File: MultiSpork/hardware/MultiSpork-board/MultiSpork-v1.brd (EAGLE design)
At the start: 86.4 x 76.2 mm, 216 parts, among them J1 U.FL, Q2 32.768 kHz, Q3 40 MHz, Q4 MMBT3904, Q5 MMBT3904, SW1 JS102011SAQN, U1 USD-SOCKETNEW, U10 M25PX80, U2 SAM3SA-MU, U3 MAX11300GTL, U4 LT3580EMS8E, U5 LT3580EMS8E, U6 LT3580EMS8E, U7 MCP73831, U8 LT3580EMS8E, U9 CC3100

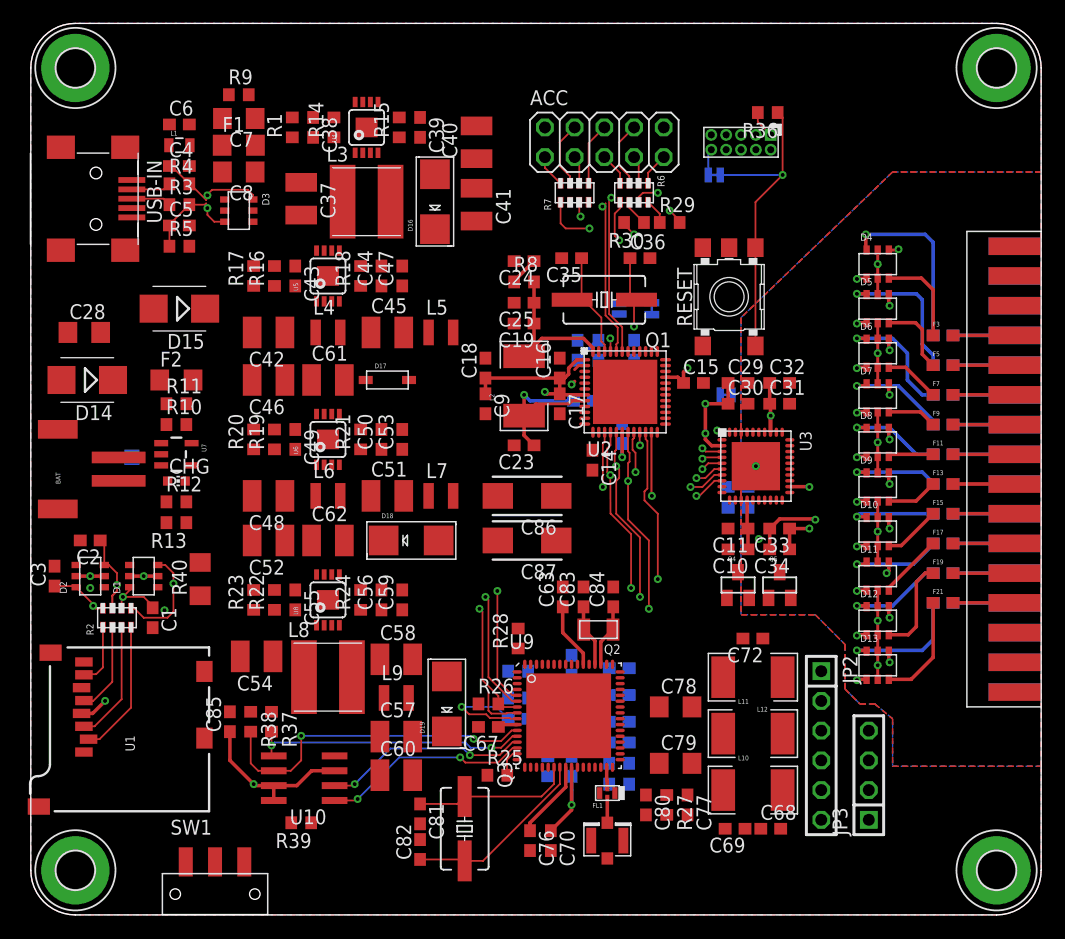
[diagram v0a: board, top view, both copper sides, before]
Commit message: Finished routing
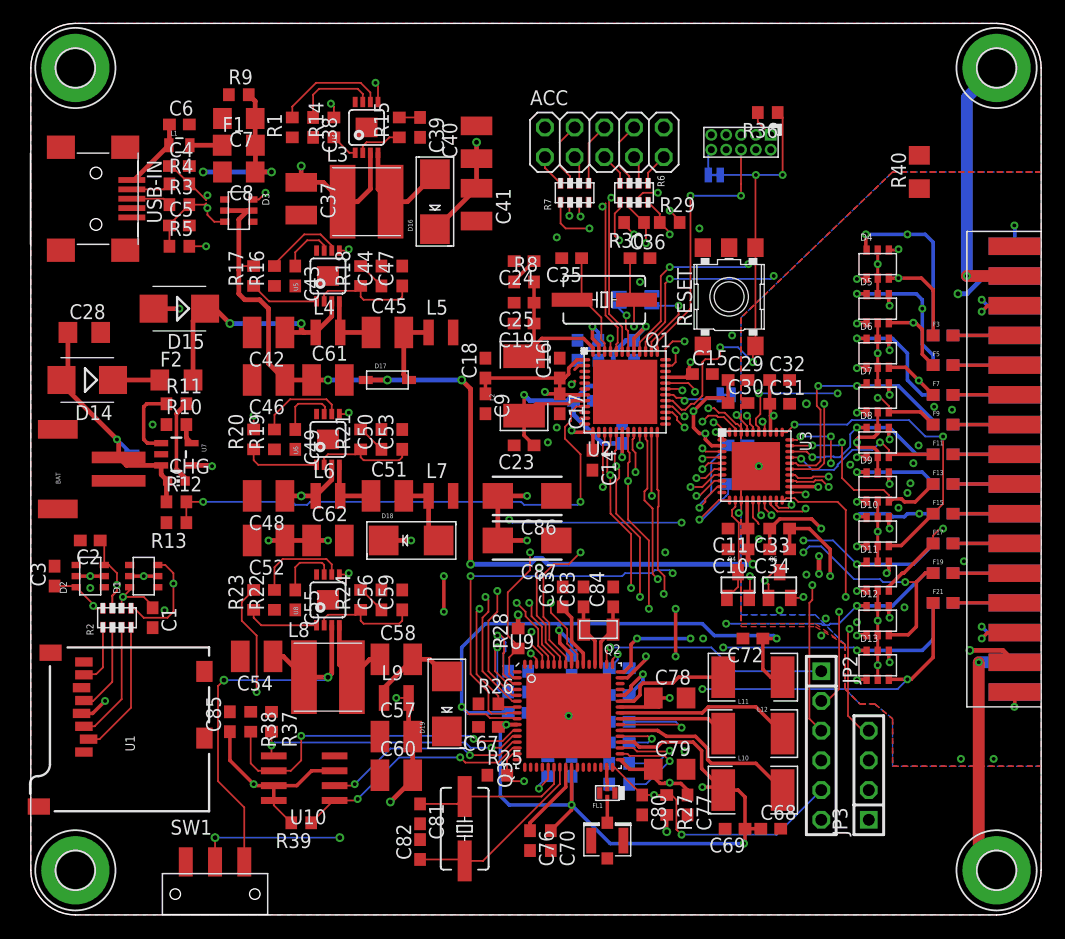
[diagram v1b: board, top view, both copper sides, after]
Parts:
- moved R40 70.6 mm to (75.9, 63.5)
- moved C21 3.56 mm to (60.5, 40.1)
- moved C27 2.03 mm to (60.5, 36.8)
- moved C15 1.08 mm to (57.4, 46.2)
- moved C78 0.92 mm to (54.6, 18.5)
- moved ERASE 0.76 mm to (50.3, 52.6)
- moved JTAGSEL 0.76 mm to (53.1, 52.6)
- moved C79 0.72 mm to (54.6, 12.4)
- moved C73 0.51 mm to (41.7, 17.3)
- moved R31 0.51 mm to (41.7, 19.1)
- moved C80 0.32 mm to (52.3, 9.40)
- moved C29 0.25 mm to (60.5, 45.7)
- moved C32 0.25 mm to (64.0, 45.7)
- moved C30 0.06 mm to (60.5, 43.8)
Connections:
- net N$115 renamed D1P
- net N$116 renamed D1N
- net N$117 renamed D0N
- net N$118 renamed D0P
- net N$19 renamed PLL-GND
- net N$32 renamed ADC_REF
- net N$33 renamed DAC_REF
- net N$34 renamed PORT00'
- net N$35 renamed PORT01'
- net N$36 renamed PORT02'
- net N$37 renamed PORT03'
- net N$38 renamed PORT04'
- net N$39 renamed PORT05'
- net N$40 renamed PORT06'
- net N$41 renamed PORT07'
- net N$42 renamed PORT08'
- net N$43 renamed PORT09'
- net N$44 renamed PORT10'
- net N$45 renamed PORT11'
- net N$46 renamed PORT12'
- net N$47 renamed PORT13'
- net N$49 renamed PORT14'
- net N$50 renamed PORT15'
- net N$51 renamed PORT16'
- net N$52 renamed PORT17'
- net N$53 renamed PORT18'
- net N$54 renamed PORT19'
- net N$56 renamed VDD_IO
- net N$79 renamed VIN_IO2
- net N$80 renamed VIN_DIG
- net N$81 renamed VIN_ANA
- net N$83 renamed VIN_PA
- net N$84 renamed ANA_SW
- net N$85 renamed VDD_PA
- net N$87 renamed PA_SWP
- net N$88 renamed PA_SWN
- net N$90 renamed VDD_DIG
- net N$92 renamed VDD_RAM
- net N$93 renamed VDD_PLL
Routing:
- net +5V: track 4.24 -> 143.4 mm, vias 0 -> 8
- net V+: track 0.00 -> 119.7 mm, vias 0 -> 6
- net SHTDWN: track 0.00 -> 86.5 mm, vias 0 -> 6
- net VDD_IO: track 10.4 -> 82.4 mm, vias 1 -> 6
- net N$99: track 0.00 -> 66.2 mm, vias 0 -> 1
- net CC_INT: track 2.42 -> 58.7 mm, vias 0 -> 4
- net CC_RST: track 0.00 -> 55.4 mm, vias 0 -> 3
- net +3V3: track 57.1 -> 112.2 mm, vias 10 -> 28
- net N$109: track 0.00 -> 54.2 mm, vias 0 -> 1
- net CC_CS: track 4.18 -> 55.4 mm, vias 0 -> 3
- net N$100: track 0.00 -> 50.7 mm, vias 0 -> 3
- net N$98: track 0.00 -> 49.1 mm, vias 0 -> 1
- net N$101: track 0.00 -> 49.1 mm, vias 0 -> 2
- net N$108: track 0.00 -> 47.2 mm, vias 0 -> 2
- net PORT18': track 9.22 -> 55.5 mm, vias 0 -> 3
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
